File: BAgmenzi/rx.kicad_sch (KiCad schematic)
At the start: 30 parts, among them IC1 TPL0501-100RSER, U2 AD8338ACPZ-R7, U3 OPA836IDBVT, U4 OPA836IDBVT

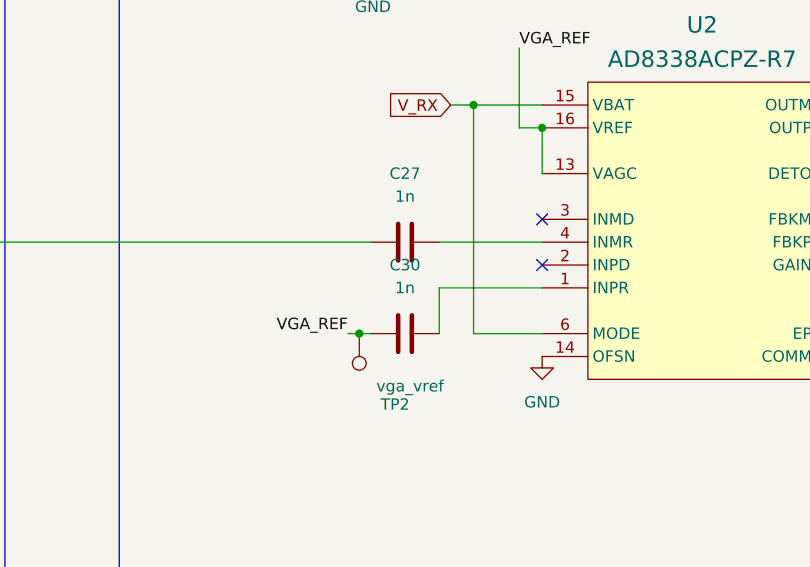
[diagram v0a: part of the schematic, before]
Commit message: powerplanes
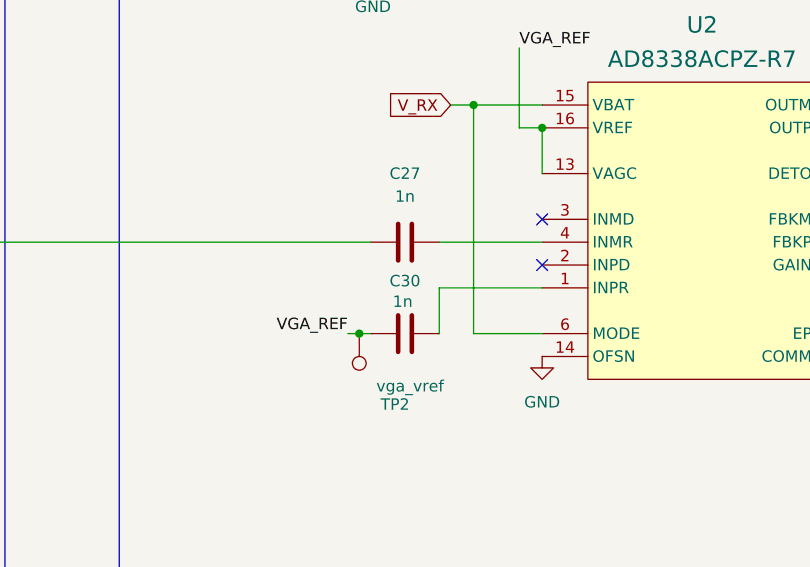
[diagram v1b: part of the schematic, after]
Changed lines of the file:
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@@
 		(on_board yes)
 		(dnp no)
-		(fields_autoplaced yes)
 		(property "Reference" "C30"
-			(at 184.15 72.39 90)
+			(at 184.15 74.168 90)
 			(effects
 				(font
@@
 		)
 		(property "Value" "1n"
-			(at 184.15 74.93 90)
+			(at 183.896 76.454 90)
 			(effects
 				(font
